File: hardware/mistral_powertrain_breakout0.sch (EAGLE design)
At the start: 24 parts, among them U1 MCP73831, U2 MCP73833-GPI/UN

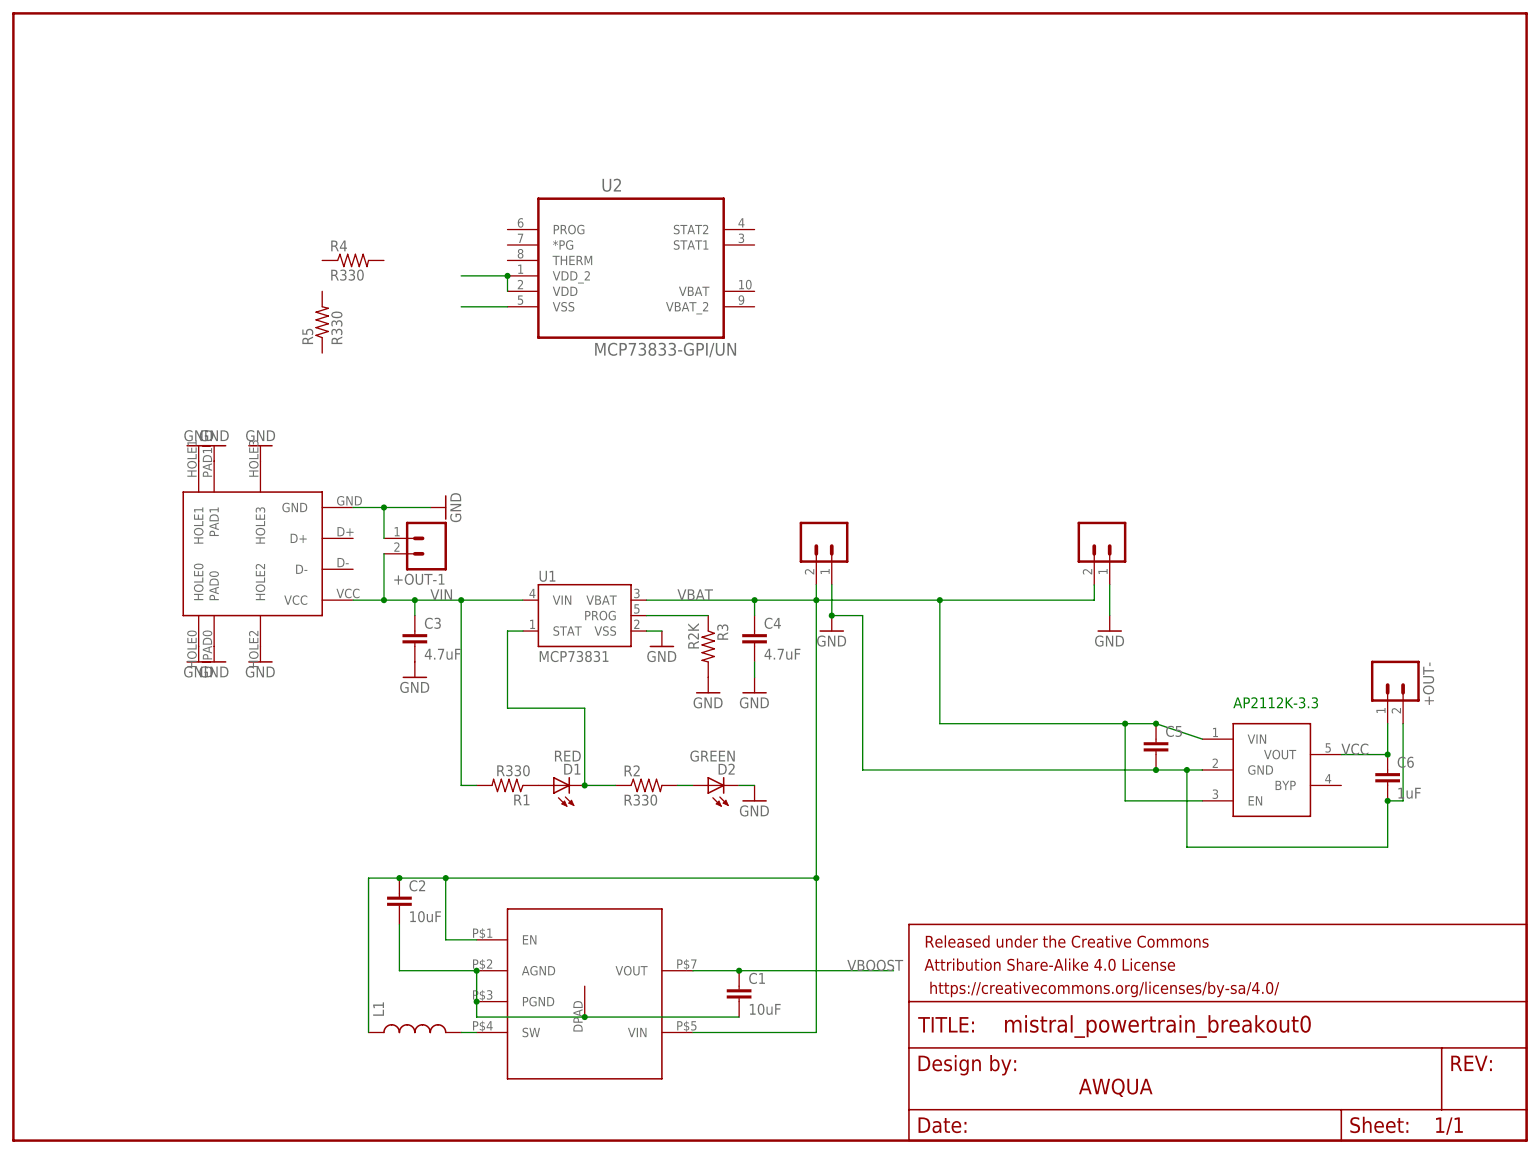
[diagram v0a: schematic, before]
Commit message: board updates
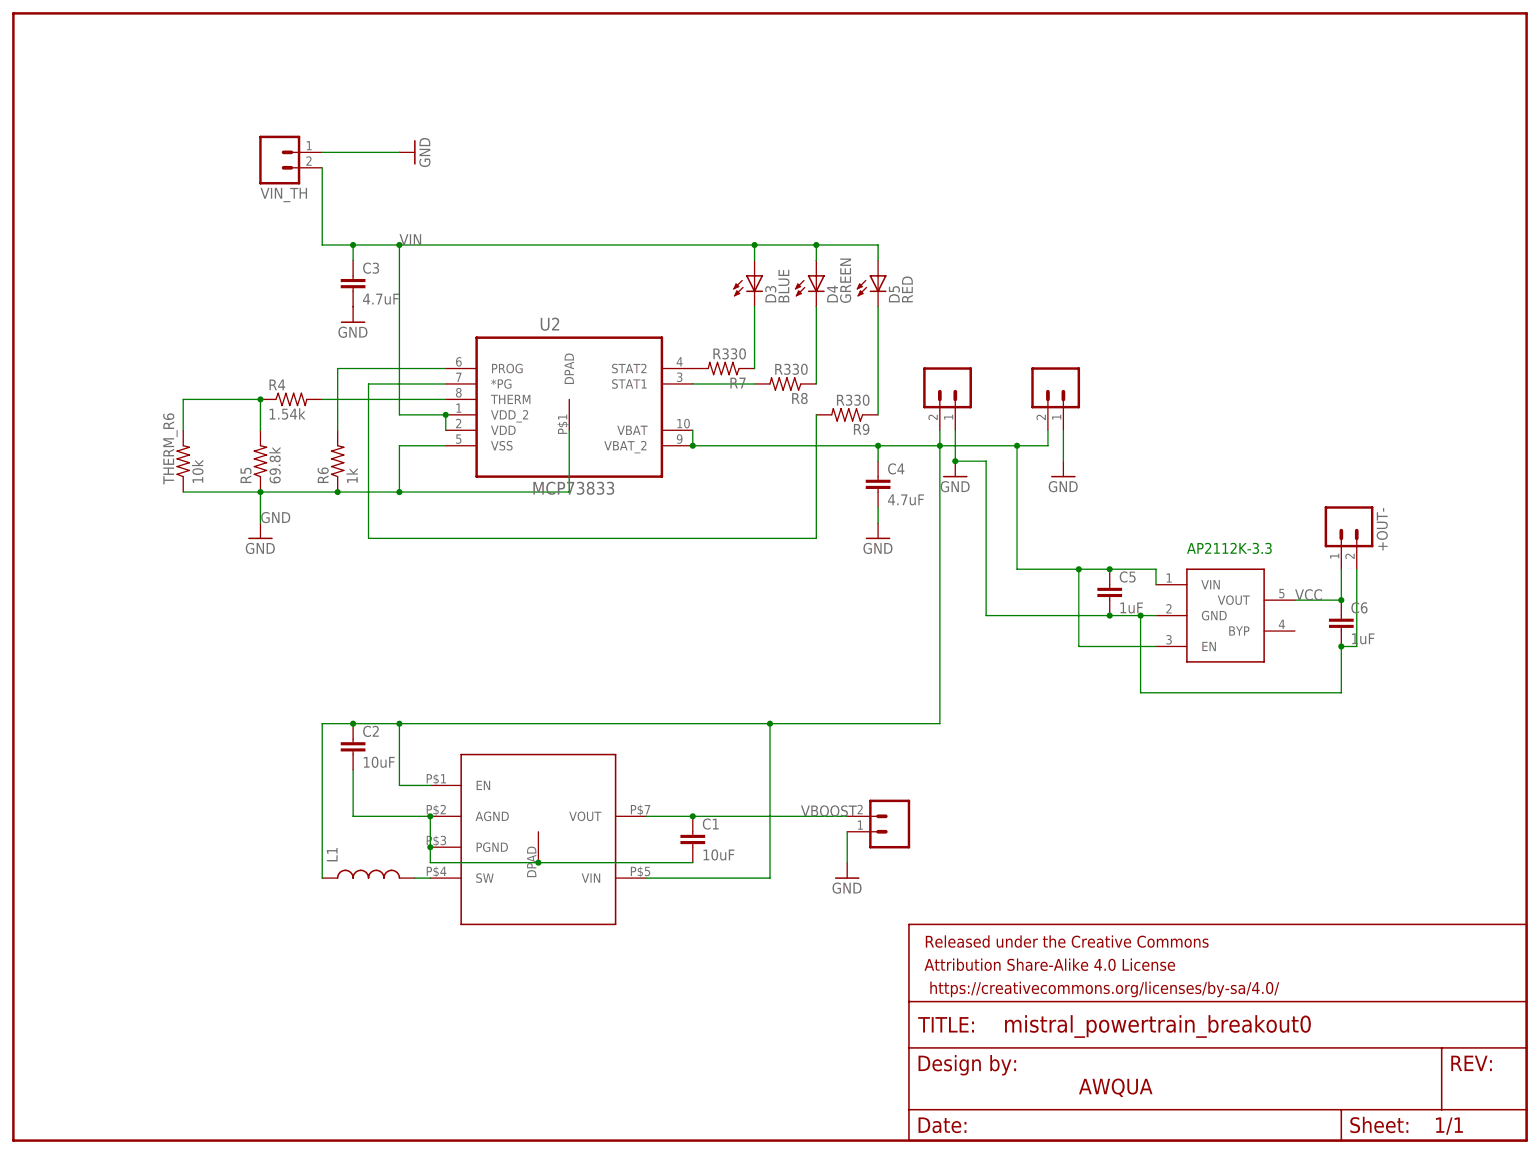
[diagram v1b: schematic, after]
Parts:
- removed +OUT-1: (no value), SparkFun-Connectors:M02PTH
- removed D1: RED, SparkFun:LED0603
- removed D2: GREEN, SparkFun:LED0603
- removed R1, R2: R330, SparkFun:RESISTOR0402-RES
- removed R3: R2K, SparkFun:RESISTOR0402-RES
- removed U$3: USBMICRO-DX4R005JJ2, awqua_eagle_library:USBMICRO-DX4R005JJ2
- removed U1: MCP73831, SparkFun:MCP73831
- added D3: BLUE, SparkFun:LED0603
- added D4: GREEN, SparkFun:LED0603
- added D5: RED, SparkFun:LED0603
- added JMP1: (no value), SparkFun:M02PTH
- added R6: 1k, SparkFun:RESISTOR0402-RES
- added R7, R8, R9: R330, SparkFun:RESISTOR0402-RES
- added THERM_R6: 10k, SparkFun:RESISTOR0402-RES
- added VIN_TH: (no value), SparkFun-Connectors:M02PTH
- C5: value (none) -> 1uF
- R4: value R330 -> 1.54k
- R5: value R330 -> 69.8k
- U2: value MCP73833-GPI/UN -> MCP73833
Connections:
- removed net N$1: U2.VDD, U2.VDD_2
- removed net N$2: D2.A, R2.2
- removed net N$3: D1.A, R1.1
- removed net N$6: U2.VSS
- removed net PROG: R3.1, U1.PROG
- removed net STAT: D1.C, R2.1, U1.STAT
- new net N$10: R7.2, U2.STAT2
- new net N$11: D3.C, R7.1
- new net N$12: R8.2, U2.STAT1
- new net N$13: D4.C, R8.1
- new net N$15: D5.C, R9.1
- new net N$16: R9.2, U2.*PG
- new net N$7: R4.2, U2.THERM
- new net N$8: R4.1, R5.2, THERM_R6.2
- new net N$9: R6.2, U2.PROG
- net GND: now also JMP1.1, R5.1, R6.1, THERM_R6.1, U2.DPAD, U2.VSS, VIN_TH.1; no longer +OUT-1.1, D2.C, R3.2, U$3.GND, U$3.HOLE0, U$3.HOLE1, U$3.HOLE2, U$3.HOLE3, U$3.PAD0, U$3.PAD1, U1.VSS
- net VBAT: now also U2.VBAT, U2.VBAT_2; no longer U1.VBAT
- net VBOOST: now also JMP1.2
- net VIN: now also D3.A, D4.A, D5.A, U2.VDD, U2.VDD_2, VIN_TH.2; no longer +OUT-1.2, R1.2, U$3.VCC, U1.VIN
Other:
- moved on the sheet: +OUT-, C1, C2, C3, C4, C5, C6, L1, R4, R5
